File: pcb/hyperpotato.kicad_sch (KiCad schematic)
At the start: 60 parts, among them J1 Conn_01x02_Socket, J2 Conn_01x02_Socket, J3 Conn_01x04, J4 Conn_01x04, J6 Conn_01x12_Socket, K1 SW_Push, K10 SW_Push, K11 SW_Push, K12 SW_Push, K13 SW_Push, K14 SW_Push, K15 SW_Push, K16 SW_Push, K17 SW_Push, K2 SW_Push, K3 SW_Push, K4 SW_Push, K5 SW_Push, K6 SW_Push, K7 SW_Push, K8 SW_Push, K9 SW_Push, SW1 SW_Push, SW2 SW_SPDT, SW3 RotaryEncoder, U1 ProMicro

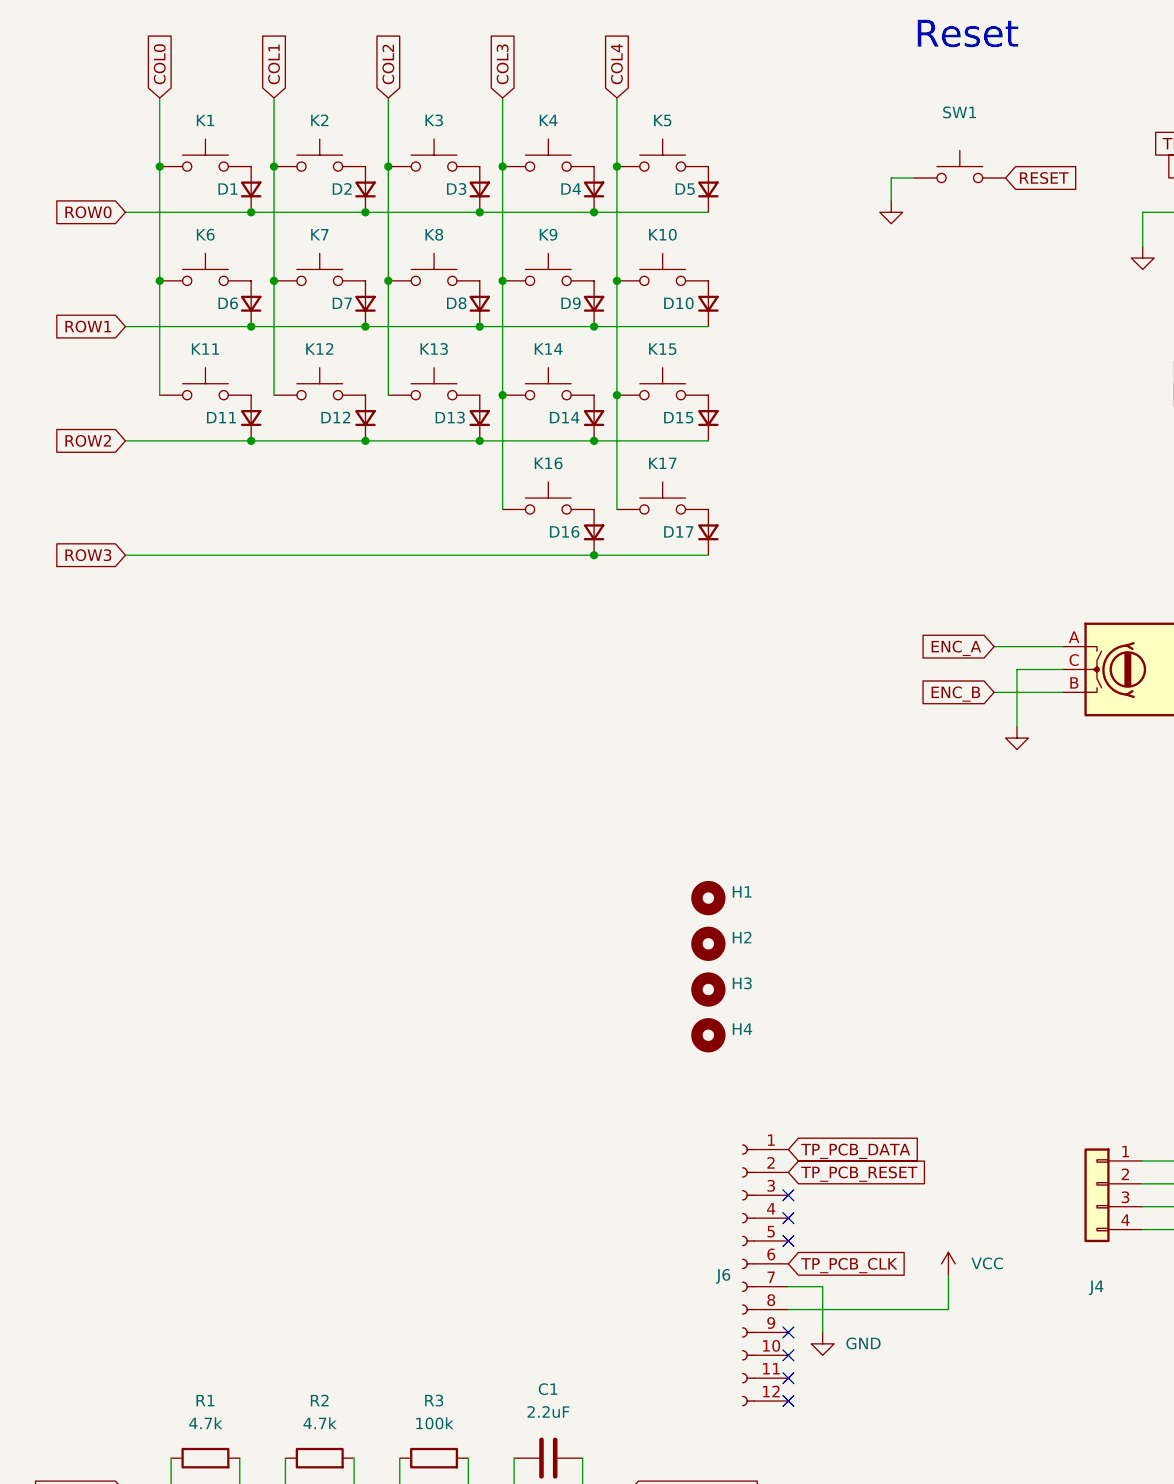
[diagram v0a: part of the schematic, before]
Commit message: WIP re-layout
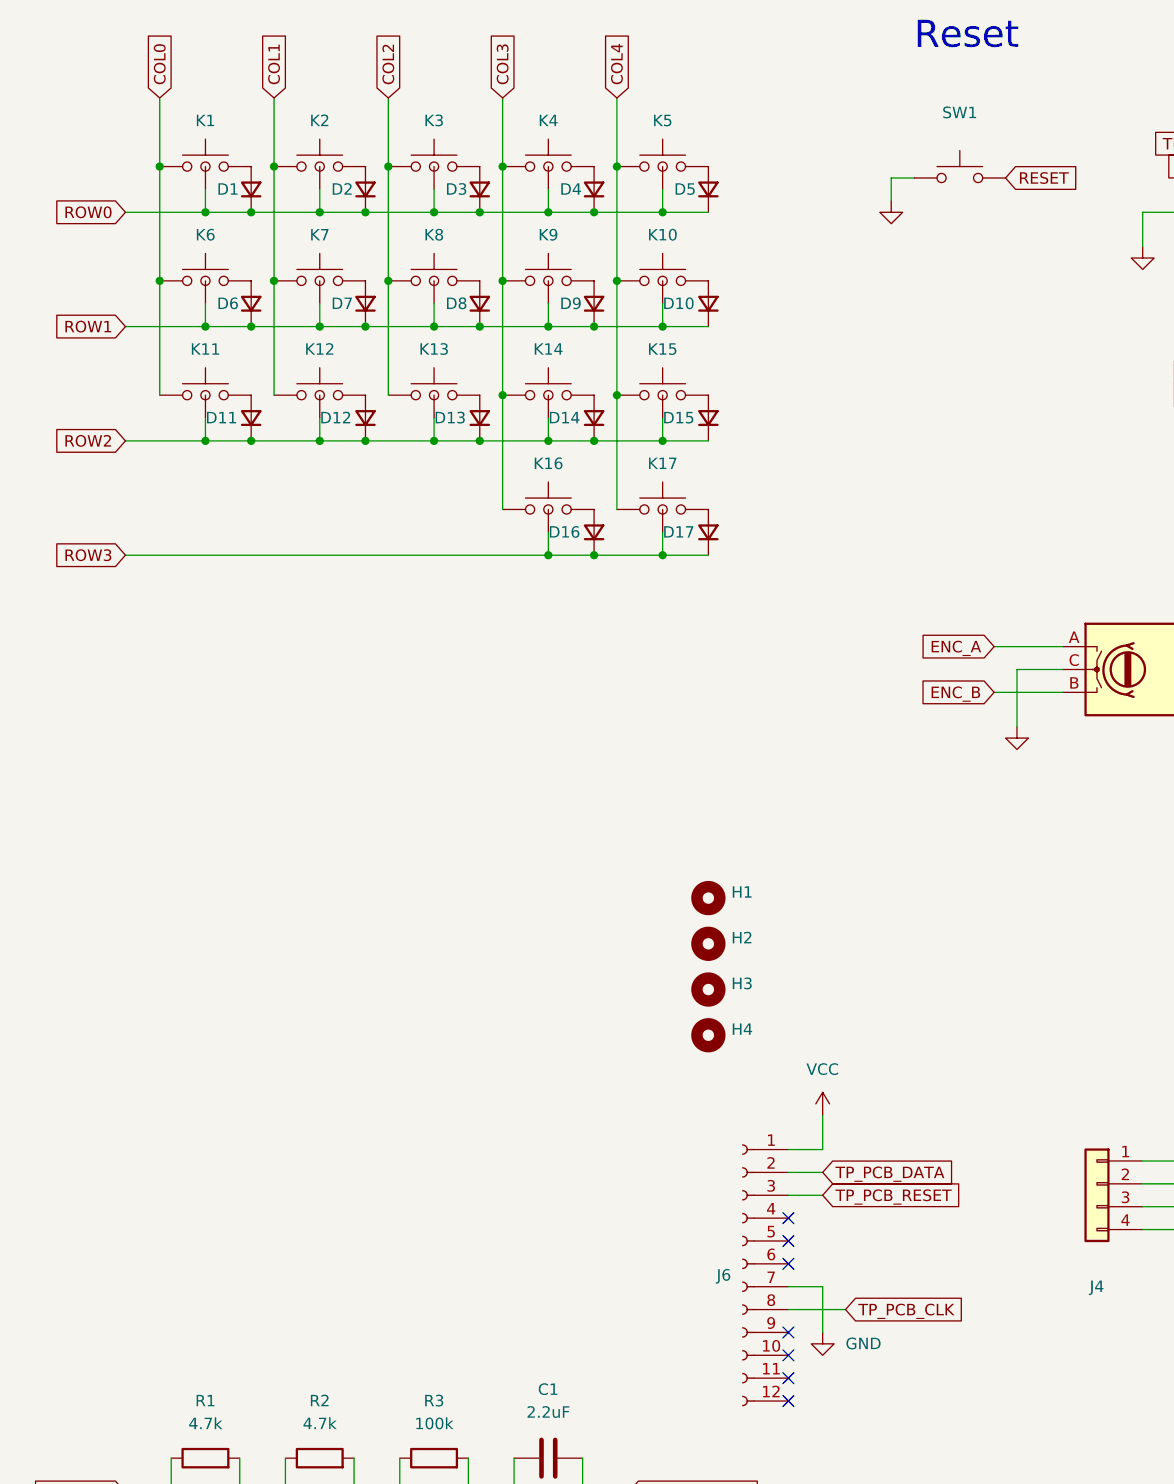
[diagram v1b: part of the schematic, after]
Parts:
- K1, K10, K11, K12, K13, K14, K16, K17, K2, K3, K4, K6, K7, K8: footprint hyperpotato:PG1350_HS_reversible_plated -> hyperpotato:V1_V2_HS_reversible_plated; symbol Switch:SW_Push -> hyperpotato:SW_Push
- K15: footprint hyperpotato:PG1350_HS_reversible_plated -> hyperpotato:V1_V2_HS_reversible_plated_alt; symbol Switch:SW_Push -> hyperpotato:SW_Push
- K5, K9: footprint hyperpotato:PG1350_reversible_side -> hyperpotato:V1_V2_HS_reversible_plated; symbol Switch:SW_Push -> hyperpotato:SW_Push
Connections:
- net COL3: now also K9.1; no longer K9.2
- net COL4: now also K15.2; no longer K15.1
- net ROW0: now also K1.3, K2.3, K3.3, K4.3, K5.3
- net ROW1: now also K10.3, K6.3, K7.3, K8.3, K9.3
- net ROW2: now also K11.3, K12.3, K13.3, K14.3, K15.3
- net ROW3: now also K16.3, K17.3
- net TP_CLK: now also J6.8 (Pin_8); no longer J6.6 (Pin_6)
- net TP_DATA: now also J6.2 (Pin_2); no longer J6.1 (Pin_1)
- net TP_PCB_RESET: now also J6.3 (Pin_3); no longer J6.2 (Pin_2)
- net VCC: now also J6.1 (Pin_1); no longer J6.8 (Pin_8)
- net at D15.2 (A): now also K15.1; no longer K15.2
- net at D9.2 (A): now also K9.2; no longer K9.1
